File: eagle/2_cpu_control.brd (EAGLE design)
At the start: 160 x 100 mm, 47 parts, among them IC1 74LS08N, IC10 74LS173N, IC11 74LS273N, IC12 74LS74N, IC13 74LS157N, IC14 74LS157N, IC15 74LS163, IC16 74LS163, IC17 74LS04N, IC2 74LS163, IC3 74LS163, IC4 74LS00N, IC5 74LS273N, IC6 74LS148N, IC7 74LS148N, IC8 74LS08N, IC9 74S32N

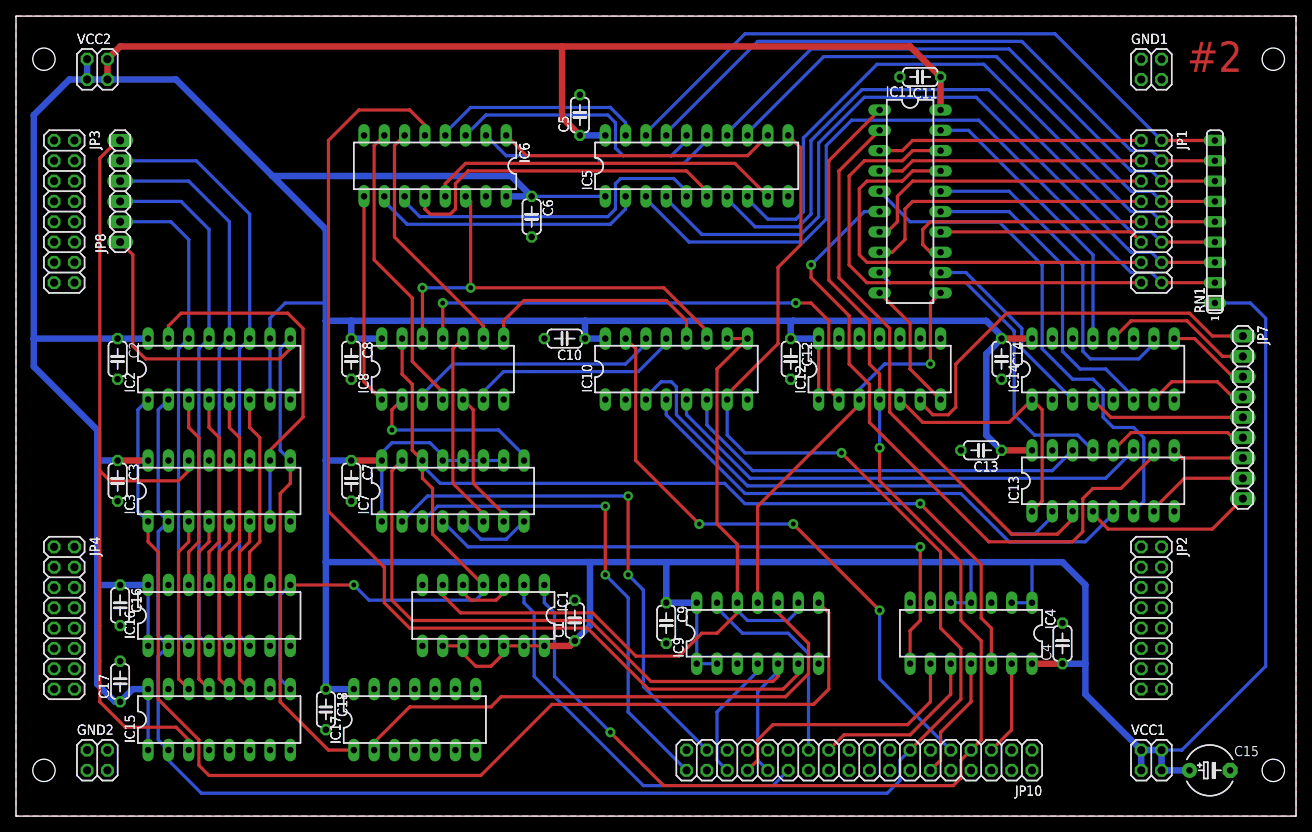
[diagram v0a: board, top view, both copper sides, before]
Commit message: 2016-02-10 17:30 (completed boards 2,6,7)
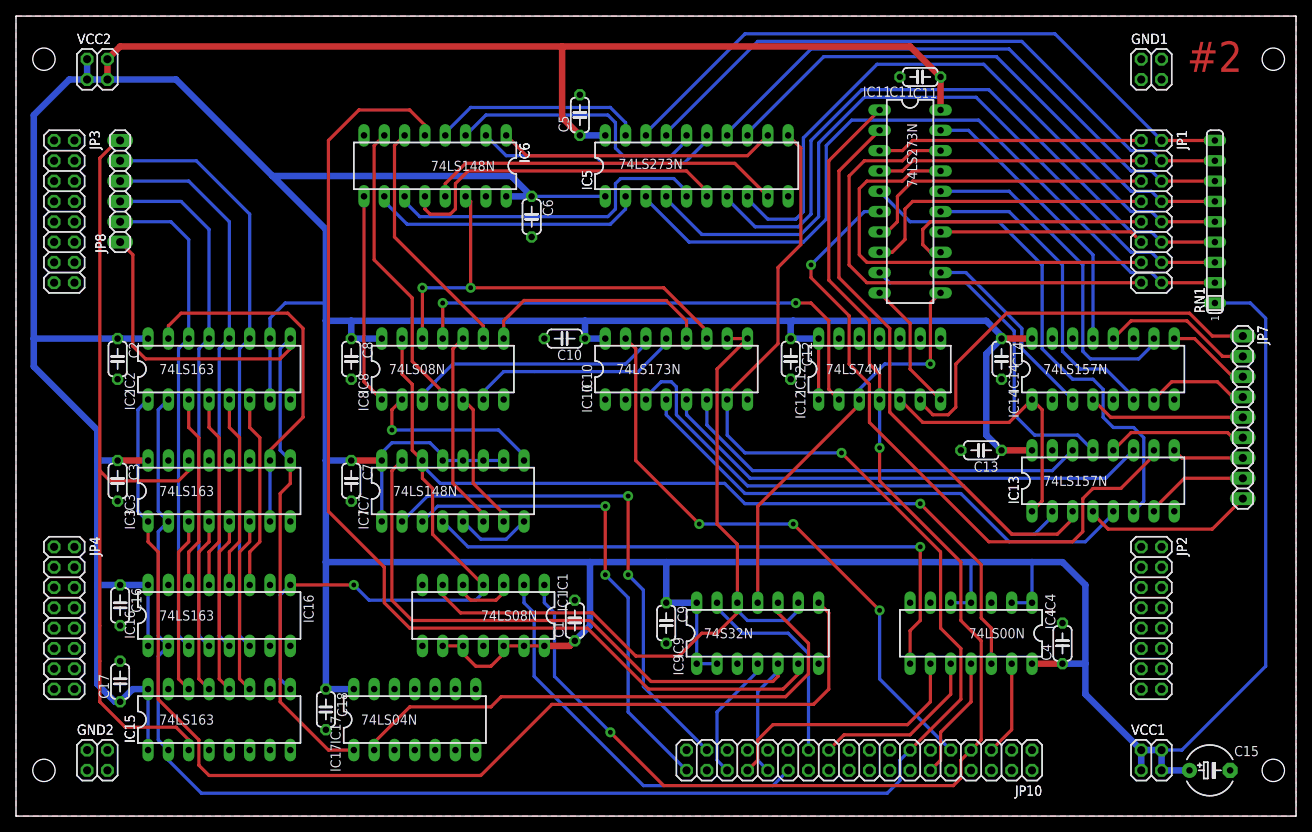
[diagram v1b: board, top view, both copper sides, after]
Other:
- board text added: "74LS00N"
- board text added: "74LS04N"
- board text added: "74LS08N"
- board text added: "74LS148N"
- board text added: "74LS157N"
- board text added: "74LS163"
- board text added: "74LS173N"
- board text added: "74LS273N"
- board text added: "74LS74N"
- board text added: "74S32N"
- board text removed: "1"
- board text removed: "C1"
- board text removed: "C10"
- board text removed: "C11"
- board text removed: "C12"
- board text removed: "C13"
- board text removed: "C14"
- board text removed: "C16"
- board text removed: "C17"
- board text removed: "C18"
- board text removed: "C3"
- board text removed: "C5"
- board text removed: "C6"
- board text removed: "C7"
- board text removed: "C8"
- board text removed: "C9"
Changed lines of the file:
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@@
 <layer number="17" name="Pads" color="2" fill="1" visible="yes" active="yes"/>
 <layer number="18" name="Vias" color="2" fill="1" visible="yes" active="yes"/>
-<layer number="19" name="Unrouted" color="6" fill="1" visible="yes" active="yes"/>
+<layer number="19" name="Unrouted" color="6" fill="1" visible="no" active="yes"/>
 <layer number="20" name="Dimension" color="15" fill="1" visible="yes" active="yes"/>
 <layer number="21" name="tPlace" color="7" fill="1" visible="no" active="yes"/>
@@
 <layer number="100" name="crosshair" color="7" fill="1" visible="no" active="yes"/>
 <layer number="121" name="tsilk" color="14" fill="1" visible="yes" active="yes"/>
-<layer number="122" name="bsilk" color="6" fill="1" visible="no" active="yes"/>
+<layer number="122" name="bsilk" color="6" fill="1" visible="yes" active="yes"/>
 </layers>
 <board>
@@
 <wire x1="150.749" y1="63.246" x2="148.971" y2="63.246" width="0.2032" layer="121"/>
 <wire x1="148.971" y1="63.246" x2="148.971" y2="65.024" width="0.2032" layer="121"/>
-<text x="150.368" y="61.849" size="0.9906" layer="121" font="vector" ratio="21" rot="R90">1</text>
 <wire x1="139.3825" y1="5.08" x2="140.0175" y2="4.445" width="0.2032" layer="121"/>
 <wire x1="141.2875" y1="4.445" x2="141.9225" y2="5.08" width="0.2032" layer="121"/>
@@
 <wire x1="10.795" y1="90.805" x2="12.065" y2="90.805" width="0.2032" layer="121"/>
 <wire x1="8.255" y1="90.805" x2="9.525" y2="90.805" width="0.2032" layer="121"/>
-<text x="68.453" y="22.2885" size="1.27" layer="121" font="vector" ratio="16" rot="R90">C1</text>
-<text x="14.097" y="44.069" size="1.27" layer="121" font="vector" ratio="16" rot="R270">C3</text>
-<text x="69.088" y="85.471" size="1.27" layer="121" font="vector" ratio="16" rot="R90">C5</text>
-<text x="65.8495" y="77.089" size="1.27" layer="121" font="vector" ratio="16" rot="R270">C6</text>
-<text x="43.307" y="44.069" size="1.27" layer="121" font="vector" ratio="16" rot="R270">C7</text>
-<text x="43.307" y="59.309" size="1.27" layer="121" font="vector" ratio="16" rot="R270">C8</text>
-<text x="82.677" y="26.289" size="1.27" layer="121" font="vector" ratio="16" rot="R270">C9</text>
-<text x="70.739" y="58.293" size="1.27" layer="121" font="vector" ratio="16" rot="R180">C10</text>
-<text x="115.189" y="90.9955" size="1.27" layer="121" font="vector" ratio="16" rot="R180">C11</text>
-<text x="98.2345" y="59.309" size="1.27" layer="121" font="vector" ratio="16" rot="R270">C12</text>
-<text x="122.809" y="44.323" size="1.27" layer="121" font="vector" ratio="16" rot="R180">C13</text>
-<text x="124.587" y="59.309" size="1.27" layer="121" font="vector" ratio="16" rot="R270">C14</text>
-<text x="14.4145" y="28.5115" size="1.27" layer="121" font="vector" ratio="16" rot="R270">C16</text>
-<text x="11.6205" y="14.6685" size="1.27" layer="121" font="vector" ratio="16" rot="R90">C17</text>
-<text x="40.132" y="15.494" size="1.27" layer="121" font="vector" ratio="16" rot="R270">C18</text>
 <text x="139.3825" y="96.52" size="1.27" layer="121" font="vector" ratio="16">GND1</text>
 <text x="7.62" y="10.16" size="1.27" layer="121" font="vector" ratio="16">GND2</text>
-<text x="67.691" y="28.1305" size="1.27" layer="121" font="vector" ratio="16" rot="R270">IC1</text>
-<text x="14.859" y="52.959" size="1.27" layer="121" font="vector" ratio="16" rot="R90">IC2</text>
-<text x="14.859" y="37.719" size="1.27" layer="121" font="vector" ratio="16" rot="R90">IC3</text>
-<text x="128.651" y="25.908" size="1.27" layer="121" font="vector" ratio="16" rot="R270">IC4</text>
+<text x="67.691" y="30.353" size="1.27" layer="121" font="vector" ratio="16" rot="R270">IC1</text>
+<text x="14.859" y="50.7365" size="1.27" layer="121" font="vector" ratio="16" rot="R90">IC2</text>
+<text x="14.859" y="35.814" size="1.27" layer="121" font="vector" ratio="16" rot="R90">IC3</text>
+<text x="128.651" y="27.813" size="1.27" layer="121" font="vector" ratio="16" rot="R270">IC4</text>
 <text x="72.009" y="78.232" size="1.27" layer="121" font="vector" ratio="16" rot="R90">IC5</text>
 <text x="62.9285" y="84.201" size="1.27" layer="121" font="vector" ratio="16" rot="R270">IC6</text>
-<text x="44.069" y="37.719" size="1.27" layer="121" font="vector" ratio="16" rot="R90">IC7</text>
-<text x="44.069" y="52.832" size="1.27" layer="121" font="vector" ratio="16" rot="R90">IC8</text>
-<text x="83.439" y="19.812" size="1.27" layer="121" font="vector" ratio="16" rot="R90">IC9</text>
-<text x="72.009" y="52.959" size="1.27" layer="121" font="vector" ratio="16" rot="R90">IC10</text>
-<text x="108.712" y="89.916" size="1.27" layer="121" font="vector" ratio="16">IC11</text>
-<text x="98.679" y="52.832" size="1.27" layer="121" font="vector" ratio="16" rot="R90">IC12</text>
+<text x="44.069" y="35.814" size="1.27" layer="121" font="vector" ratio="16" rot="R90">IC7</text>
+<text x="44.069" y="50.6095" size="1.27" layer="121" font="vector" ratio="16" rot="R90">IC8</text>
+<text x="83.439" y="17.5895" size="1.27" layer="121" font="vector" ratio="16" rot="R90">IC9</text>
+<text x="72.009" y="50.419" size="1.27" layer="121" font="vector" ratio="16" rot="R90">IC10</text>
+<text x="105.8545" y="89.916" size="1.27" layer="121" font="vector" ratio="16">IC11</text>
+<text x="98.679" y="49.657" size="1.27" layer="121" font="vector" ratio="16" rot="R90">IC12</text>
 <text x="125.349" y="38.989" size="1.27" layer="121" font="vector" ratio="16" rot="R90">IC13</text>
-<text x="125.349" y="52.959" size="1.27" layer="121" font="vector" ratio="16" rot="R90">IC14</text>
+<text x="125.349" y="49.784" size="1.27" layer="121" font="vector" ratio="16" rot="R90">IC14</text>
 <text x="14.859" y="9.144" size="1.27" layer="121" font="vector" ratio="16" rot="R90">IC15</text>
-<text x="14.859" y="22.1615" size="1.27" layer="121" font="vector" ratio="16" rot="R90">IC16</text>
-<text x="40.5765" y="9.017" size="1.27" layer="121" font="vector" ratio="16" rot="R90">IC17</text>
+<text x="35.941" y="27.686" size="1.27" layer="121" font="vector" ratio="16" rot="R270">IC16</text>
+<text x="40.5765" y="5.5245" size="1.27" layer="121" font="vector" ratio="16" rot="R90">IC17</text>
 <text x="145.0975" y="85.725" size="1.27" layer="121" font="vector" ratio="16" rot="R270">JP1</text>
 <text x="145.0975" y="34.925" size="1.27" layer="121" font="vector" ratio="16" rot="R270">JP2</text>
@@
 <text x="139.3825" y="10.16" size="1.27" layer="121" font="vector" ratio="16">VCC1</text>
 <text x="7.62" y="96.52" size="1.27" layer="121" font="vector" ratio="16">VCC2</text>
+<text x="65.151" y="25.7175" size="1.27" layer="121" font="vector" ratio="16" rot="R180">74LS08N</text>
+<text x="17.907" y="55.245" size="1.27" layer="121" font="vector" ratio="16">74LS163</text>
+<text x="17.907" y="40.005" size="1.27" layer="121" font="vector" ratio="16">74LS163</text>
+<text x="126.111" y="23.495" size="1.27" layer="121" font="vector" ratio="16" rot="R180">74LS00N</text>
+<text x="75.311" y="80.899" size="1.27" layer="121" font="vector" ratio="16">74LS273N</text>
+<text x="59.8805" y="81.915" size="1.27" layer="121" font="vector" ratio="16" rot="R180">74LS148N</text>
+<text x="47.117" y="40.005" size="1.27" layer="121" font="vector" ratio="16">74LS148N</text>
+<text x="46.609" y="55.245" size="1.27" layer="121" font="vector" ratio="16">74LS08N</text>
+<text x="85.979" y="22.225" size="1.27" layer="121" font="vector" ratio="16">74S32N</text>
+<text x="75.057" y="55.245" size="1.27" layer="121" font="vector" ratio="16">74LS173N</text>
+<text x="111.379" y="86.614" size="1.27" layer="121" font="vector" ratio="16" rot="R270">74LS273N</text>
+<text x="101.219" y="55.245" size="1.27" layer="121" font="vector" ratio="16">74LS74N</text>
+<text x="128.397" y="41.275" size="1.27" layer="121" font="vector" ratio="16">74LS157N</text>
+<text x="128.397" y="55.245" size="1.27" layer="121" font="vector" ratio="16">74LS157N</text>
+<text x="17.907" y="11.43" size="1.27" layer="121" font="vector" ratio="16">74LS163</text>
+<text x="17.907" y="24.4475" size="1.27" layer="121" font="vector" ratio="16">74LS163</text>
+<text x="43.1165" y="11.43" size="1.27" layer="121" font="vector" ratio="16">74LS04N</text>
 </plain>
 <attributes>
@@
 <wire x1="73.66" y1="30.1625" x2="76.5175" y2="27.305" width="0.4064" layer="16"/>
 <wire x1="76.5175" y1="27.305" x2="76.5175" y2="13.0175" width="0.4064" layer="16"/>
-<via x="73.66" y="38.735" extent="1-16" drill="0.6096"/>
-<via x="73.66" y="30.1625" extent="1-16" drill="0.6096"/>
+<via x="73.66" y="38.735" extent="1-16" drill="0.6096" diameter="1.27"/>
+<via x="73.66" y="30.1625" extent="1-16" drill="0.6096" diameter="1.27"/>
 <wire x1="83.82" y1="5.715" x2="76.5175" y2="13.0175" width="0.4064" layer="16"/>
 </signal>
@@
 <wire x1="76.5175" y1="30.1625" x2="78.4225" y2="28.2575" width="0.4064" layer="16"/>
 <wire x1="78.4225" y1="28.2575" x2="78.4225" y2="16.1925" width="0.4064" layer="16"/>
-<via x="76.5175" y="40.005" extent="1-16" drill="0.6096"/>
-<via x="76.5175" y="30.1625" extent="1-16" drill="0.6096"/>
+<via x="76.5175" y="40.005" extent="1-16" drill="0.6096" diameter="1.27"/>
+<via x="76.5175" y="30.1625" extent="1-16" drill="0.6096" diameter="1.27"/>
 <wire x1="86.36" y1="8.255" x2="78.4225" y2="16.1925" width="0.4064" layer="16"/>
 </signal>
@@
 <wire x1="114.3" y1="56.515" x2="114.3" y2="64.135" width="0.4064" layer="1"/>
 <wire x1="114.3" y1="64.135" x2="115.57" y2="65.405" width="0.4064" layer="1"/>
-<via x="114.3" y="56.515" extent="1-16" drill="0.6096"/>
+<via x="114.3" y="56.515" extent="1-16" drill="0.6096" diameter="1.27"/>
 <wire x1="92.71" y1="26.67" x2="92.71" y2="38.735" width="0.4064" layer="1"/>
 <wire x1="92.71" y1="38.735" x2="105.41" y2="51.435" width="0.4064" layer="1"/>
